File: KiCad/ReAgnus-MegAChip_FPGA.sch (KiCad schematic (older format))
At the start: 3 parts, among them J2 Conn_02x05_Odd_Even, U7 GW1N-UV9LQ144

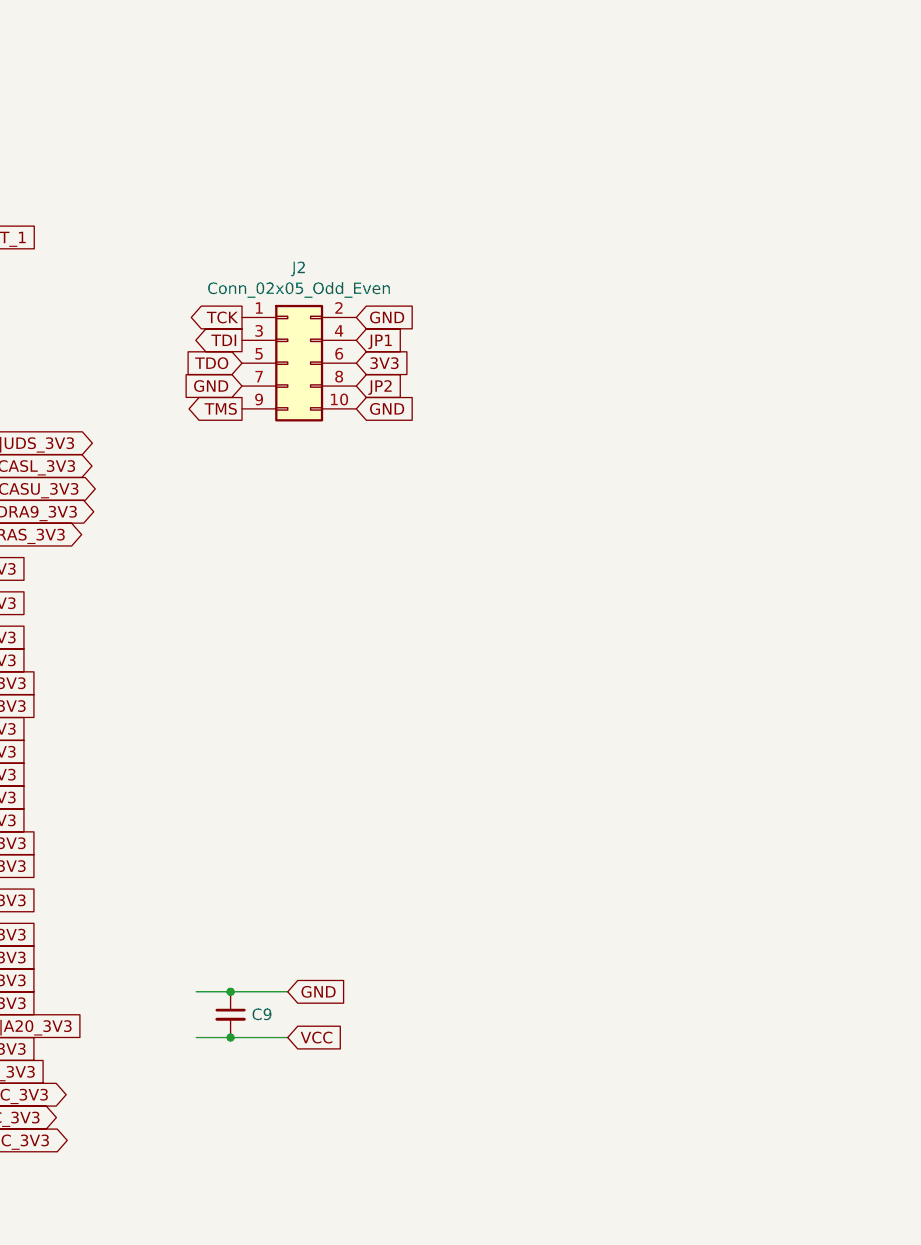
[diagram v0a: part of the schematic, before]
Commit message: more routing and placing components
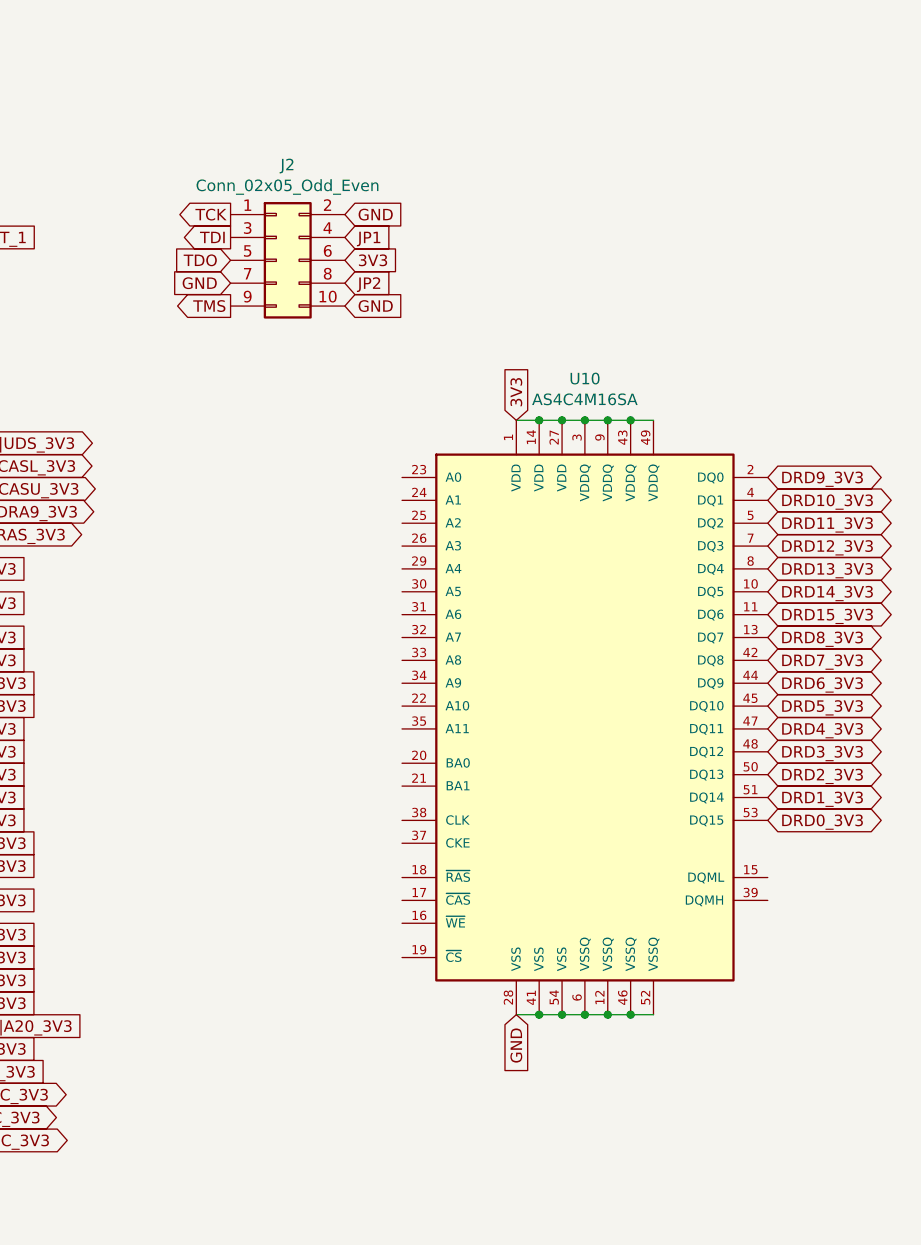
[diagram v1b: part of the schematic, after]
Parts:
- removed C9: C_Small, Capacitor_SMD:C_1206_3216Metric_Pad1.42x1.75mm_HandSolder, symbol Device:C_Small
- added U10: AS4C4M16SA, Package_SO:TSOP-II-54_22.2x10.16mm_P0.8mm, symbol Memory_RAM:AS4C4M16SA
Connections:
- net labels removed: VCC
- wire segments 25 -> 33
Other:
- moved on the sheet: J2
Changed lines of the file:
@@
 Comment4 ""
 $EndDescr
-Text GLabel 7850 5100 2    50   Input ~ 0
-VCC
-Text GLabel 7850 4900 2    50   Input ~ 0
-GND
 Text GLabel 3900 4400 3    50   Input ~ 0
 GND
-$Comp
-L Device:C_Small C?
-U 1 1 632F85C6
-P 7600 5000
-AR Path="/632F85C6" Ref="C?"  Part="1"
-AR Path="/632D3BDF/632F85C6" Ref="C?"  Part="1"
-AR Path="/632F104D/632F85C6" Ref="C9"  Part="1"
-F 0 "C9" H 7692 5000 50  0000 L CNN
-F 1 "C_Small" H 7692 4955 50  0001 L CNN
-F 2 "Capacitor_SMD:C_1206_3216Metric_Pad1.42x1.75mm_HandSolder" H 7600 5000 50  0001 C CNN
-F 3 "~" H 7600 5000 50  0001 C CNN
-	1    7600 5000
-	1    0    0    -1
-$EndComp
-Wire Wire Line
-	7450 4900 7600 4900
-Connection ~ 7600 4900
-Wire Wire Line
-	7600 4900 7850 4900
-Wire Wire Line
-	7450 5100 7600 5100
-Connection ~ 7600 5100
-Wire Wire Line
-	7600 5100 7850 5100
 Text GLabel 3200 1050 1    50   Input ~ 0
 3V3
@@
 L Connector_Generic:Conn_02x05_Odd_Even J2
 U 1 1 6329A00B
-P 7850 2150
-F 0 "J2" H 7900 2567 50  0000 C CNN
-F 1 "Conn_02x05_Odd_Even" H 7900 2476 50  0000 C CNN
-F 2 "Connector_PinHeader_2.54mm:PinHeader_2x05_P2.54mm_Vertical" H 7850 2150 50  0001 C CNN
-F 3 "~" H 7850 2150 50  0001 C CNN
-	1    7850 2150
+P 7800 1700
+F 0 "J2" H 7850 2117 50  0000 C CNN
+F 1 "Conn_02x05_Odd_Even" H 7850 2026 50  0000 C CNN
+F 2 "Connector_PinHeader_2.54mm:PinHeader_2x05_P2.54mm_Vertical" H 7800 1700 50  0001 C CNN
+F 3 "~" H 7800 1700 50  0001 C CNN
+	1    7800 1700
 	1    0    0    -1
 $EndComp
-Text GLabel 7650 1950 0    50   Output ~ 0
+Text GLabel 7600 1500 0    50   Output ~ 0
 TCK
-Text GLabel 7650 2050 0    50   Output ~ 0
+Text GLabel 7600 1600 0    50   Output ~ 0
 TDI
-Text GLabel 7650 2150 0    50   Input ~ 0
+Text GLabel 7600 1700 0    50   Input ~ 0
 TDO
-Text GLabel 7650 2250 0    50   Input ~ 0
-GND
-Text GLabel 7650 2350 0    50   Output ~ 0
+Text GLabel 7600 1800 0    50   Input ~ 0
+GND
+Text GLabel 7600 1900 0    50   Output ~ 0
 TMS
-Text GLabel 8150 1950 2    50   Input ~ 0
-GND
-Text GLabel 8150 2350 2    50   Input ~ 0
-GND
-Text GLabel 8150 2050 2    50   Input ~ 0
+Text GLabel 8100 1500 2    50   Input ~ 0
+GND
+Text GLabel 8100 1900 2    50   Input ~ 0
+GND
+Text GLabel 8100 1600 2    50   Input ~ 0
 JP1
-Text GLabel 8150 2250 2    50   Input ~ 0
+Text GLabel 8100 1800 2    50   Input ~ 0
 JP2
-Text GLabel 8150 2150 2    50   Input ~ 0
+Text GLabel 8100 1700 2    50   Input ~ 0
 3V3
 Text GLabel 1450 3400 0    50   Input ~ 0
@@
 MODE0
 NoConn ~ 1450 2450
+$Comp
+L Memory_RAM:AS4C4M16SA U10
+U 1 1 632B4228
+P 9150 3700
+F 0 "U10" H 9150 5181 50  0000 C CNN
+F 1 "AS4C4M16SA" H 9150 5090 50  0000 C CNN
+F 2 "Package_SO:TSOP-II-54_22.2x10.16mm_P0.8mm" H 9150 3700 50  0001 C CIN
+F 3 "https://www.alliancememory.com/wp-content/uploads/pdf/dram/64M-AS4C4M16SA-CI_v3.0_March%202015.pdf" H 9150 3450 50  0001 C CNN
+	1    9150 3700
+	1    0    0    -1
+$EndComp
+Text GLabel 9950 4150 2    50   BiDi ~ 0
+DRD0_3V3
+Text GLabel 9950 4050 2    50   BiDi ~ 0
+DRD1_3V3
+Text GLabel 9950 3950 2    50   BiDi ~ 0
+DRD2_3V3
+Text GLabel 9950 3850 2    50   BiDi ~ 0
+DRD3_3V3
+Text GLabel 9950 3750 2    50   BiDi ~ 0
+DRD4_3V3
+Text GLabel 9950 3650 2    50   BiDi ~ 0
+DRD5_3V3
+Text GLabel 9950 3550 2    50   BiDi ~ 0
+DRD6_3V3
+Text GLabel 9950 3450 2    50   BiDi ~ 0
+DRD7_3V3
+Text GLabel 9950 3350 2    50   BiDi ~ 0
+DRD8_3V3
+Text GLabel 9950 2650 2    50   BiDi ~ 0
+DRD9_3V3
+Text GLabel 9950 2750 2    50   BiDi ~ 0
+DRD10_3V3
+Text GLabel 9950 2850 2    50   BiDi ~ 0
+DRD11_3V3
+Text GLabel 9950 2950 2    50   BiDi ~ 0
+DRD12_3V3
+Text GLabel 9950 3050 2    50   BiDi ~ 0
+DRD13_3V3
+Text GLabel 9950 3150 2    50   BiDi ~ 0
+DRD14_3V3
+Text GLabel 9950 3250 2    50   BiDi ~ 0
+DRD15_3V3
+Text GLabel 8850 2400 1    50   Input ~ 0
+3V3
+Wire Wire Line
+	8850 2400 8950 2400
+Connection ~ 8950 2400
+Wire Wire Line
+	8950 2400 9050 2400
+Connection ~ 9050 2400
+Wire Wire Line
+	9050 2400 9150 2400
+Connection ~ 9150 2400
+Wire Wire Line
+	9150 2400 9250 2400
+Connection ~ 9250 2400
+Wire Wire Line
+	9250 2400 9350 2400
+Connection ~ 9350 2400
+Wire Wire Line
+	9350 2400 9450 2400
+Text GLabel 8850 5000 3    50   Input ~ 0
+GND
+Wire Wire Line
+	8850 5000 8950 5000
+Connection ~ 8950 5000
+Wire Wire Line
+	8950 5000 9050 5000
+Connection ~ 9050 5000
+Wire Wire Line
+	9050 5000 9150 5000
+Connection ~ 9150 5000
+Wire Wire Line
+	9150 5000 9250 5000
+Connection ~ 9250 5000
+Wire Wire Line
+	9250 5000 9350 5000
+Connection ~ 9350 5000
+Wire Wire Line
+	9350 5000 9450 5000
 $EndSCHEMATC
